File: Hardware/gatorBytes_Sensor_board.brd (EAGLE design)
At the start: 91.4 x 44.5 mm, 53 parts, among them U2 LIGHT_SENSORTEMT6000, U3 MCP9700TT

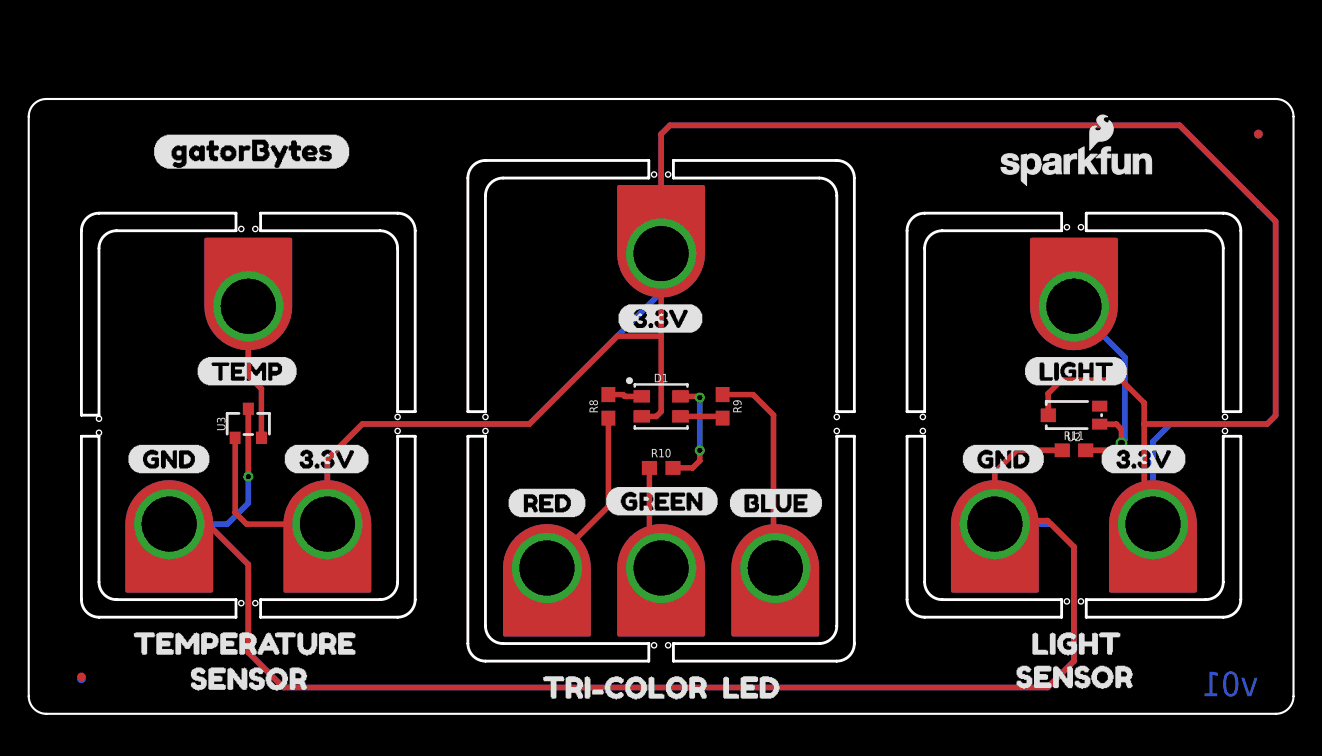
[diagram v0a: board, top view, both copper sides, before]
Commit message: adding new tabs
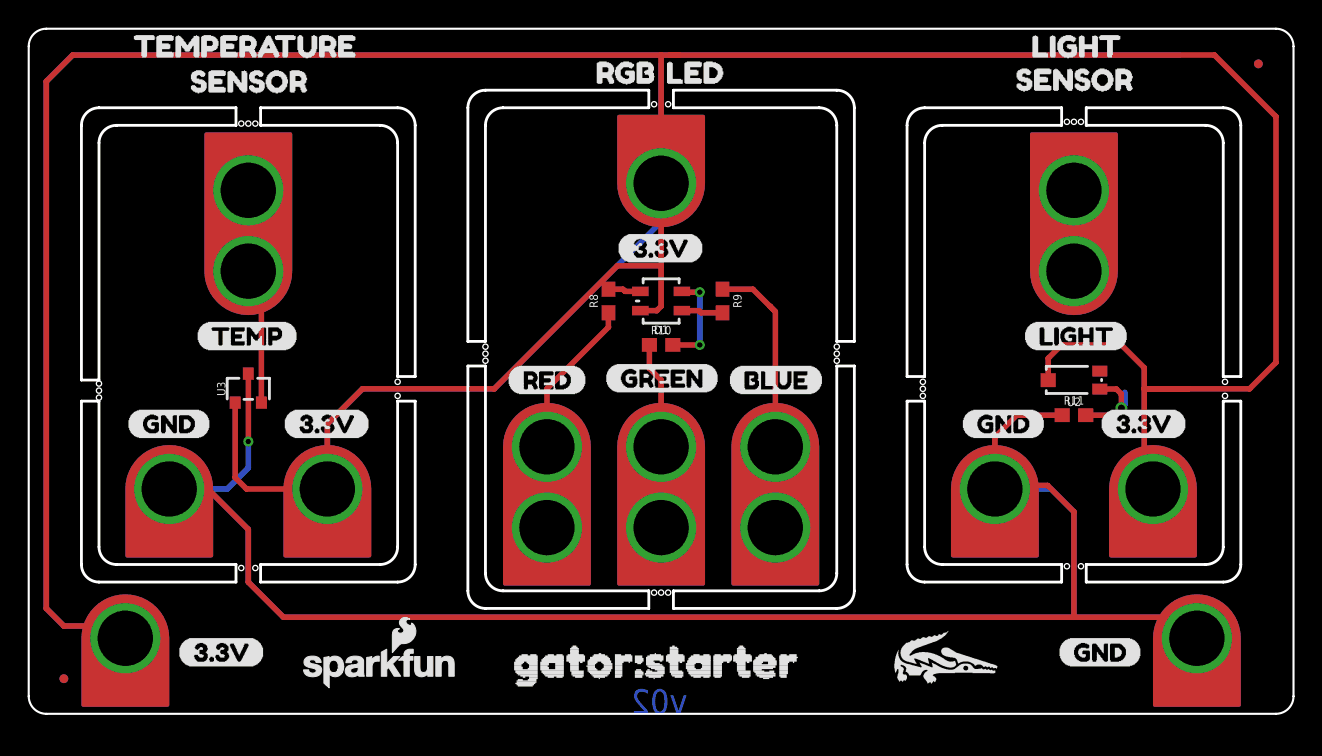
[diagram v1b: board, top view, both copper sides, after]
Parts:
- added U$35: GATOR_MINI, TAB:GATOR_MINI
- added U$36, U$37: (no value), 001:3#3V1
- added U$38, U$39: (no value), 001:GND0
- added U$40: (no value), buzzard_labels (1):RGB0
- added U$41: (no value), gator#PNG (6):GATOR#PNG
- D1: device SparkFun-LED:PLCC4SMDLED -> SparkFun-LED:LED-TRICOLOR-SMD
- U$10, U$14, U$15, U$23, U$24: value GATOR_MINI -> GATOR; device TAB:GATOR_MINI -> SparkFun-Connectors:GATOR
- U$19: value (none) -> GATOR_MINI; device 002:TRI#COLOR5 -> TAB:GATOR_MINI
- U$30: device 003:GATORBYTES6 -> buzzard_labels (4):GATOR#STARTER0
- moved U$5 62.1 mm to (19.4, 1.78)
- moved U$27 44.6 mm to (44.7, 46.4)
- moved U$30 44.0 mm to (33.0, 3.81)
- moved U$16 43.2 mm to (10.3, 45.7)
- moved U$17 43.2 mm to (6.22, 48.3)
- moved U$20 43.2 mm to (71.1, 48.3)
- moved U$21 43.2 mm to (70.0, 45.8)
- moved U$19 28.9 mm to (6.99, 0.64)
- moved U$10 13.8 mm to (37.5, 19.6)
- moved U$14 13.8 mm to (54.0, 19.6)
- moved U$15 13.8 mm to (45.7, 19.6)
- moved R10 8.89 mm to (45.7, 26.7)
- moved U$8 8.89 mm to (41.7, 24.3)
- moved U$18 8.89 mm to (34.5, 24.1)
- moved U$4 8.89 mm to (50.5, 24.1)
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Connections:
- net 3.3V: now also D1.A, U$19.P1; no longer D1.4
- net GND: now also U$35.P1
- net N$10: now also U$23.P$1, U$23.P$2; no longer U$23.P1
- net N$11: now also D1.B; no longer D1.3
- net N$12: now also D1.R; no longer D1.1
- net N$13: now also D1.G; no longer D1.2
- net N$14: now also U$10.P$1, U$10.P$2; no longer U$10.P1
- net N$15: now also U$14.P$1, U$14.P$2; no longer U$14.P1
- net N$16: now also U$15.P$1, U$15.P$2; no longer U$15.P1
- net N$18: now also U$24.P$1, U$24.P$2; no longer U$24.P1
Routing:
- net 3.3V: track 279.0 -> 428.0 mm
- net GND: track 200.6 -> 211.7 mm
- net N$18: track 17.1 -> 6.76 mm
- net N$10: track 9.90 -> 16.3 mm
- net N$14: track 12.7 -> 11.5 mm
- net N$13: track 8.16 -> 7.07 mm
- net N$15: track 15.4 -> 14.7 mm
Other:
- board size 91.4 x 44.5 mm -> 91.4 x 49.5 mm
- board text added: "v02"
- board text removed: "v01"
